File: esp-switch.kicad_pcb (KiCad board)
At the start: 2 copper layers, 50.8 x 50.8 mm, 29 parts, among them J1 Screw_Terminal_01x03, J2 Conn_01x04, J3 Screw_Terminal_01x03, J4 Conn_01x04, U1 ATTINY441-SSU, U2 ESP-01v090, U3 MOC3041M, U4 MOC3041M, U5 HLK-PM03

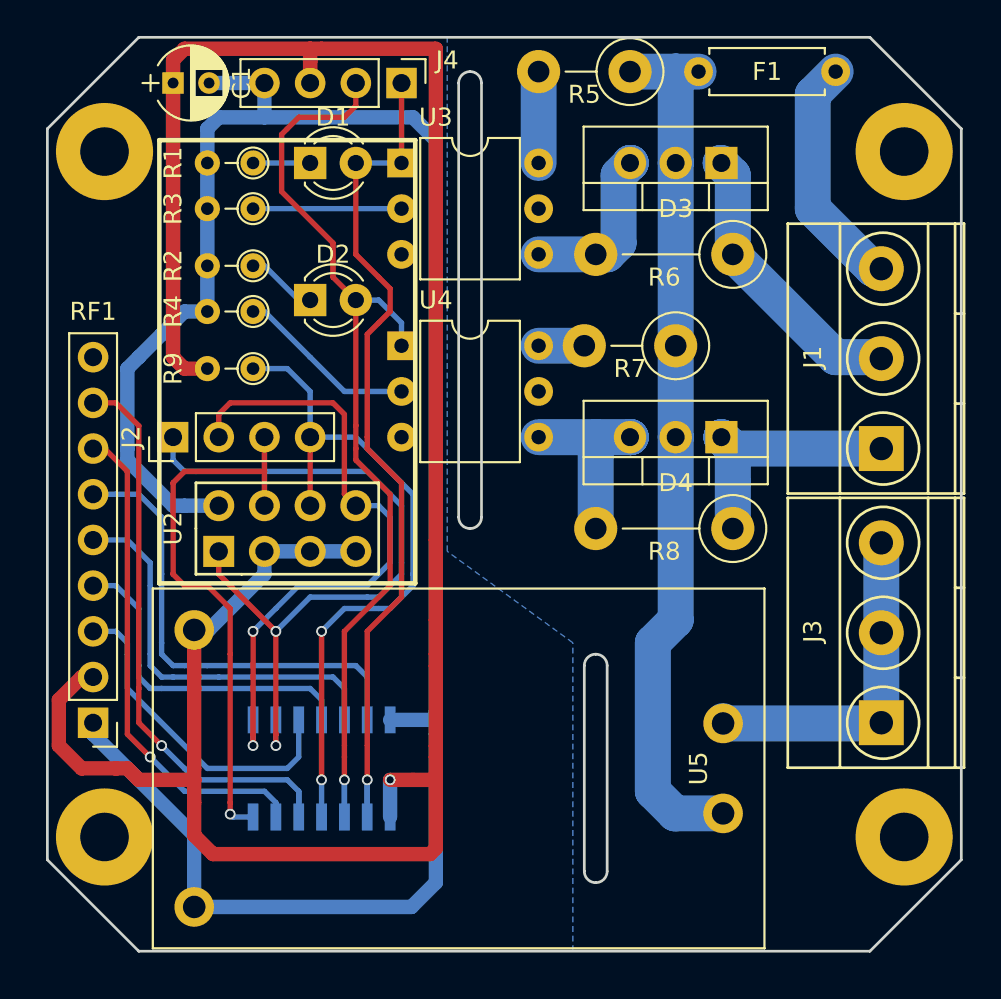
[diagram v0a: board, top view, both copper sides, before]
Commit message: V4 schematics
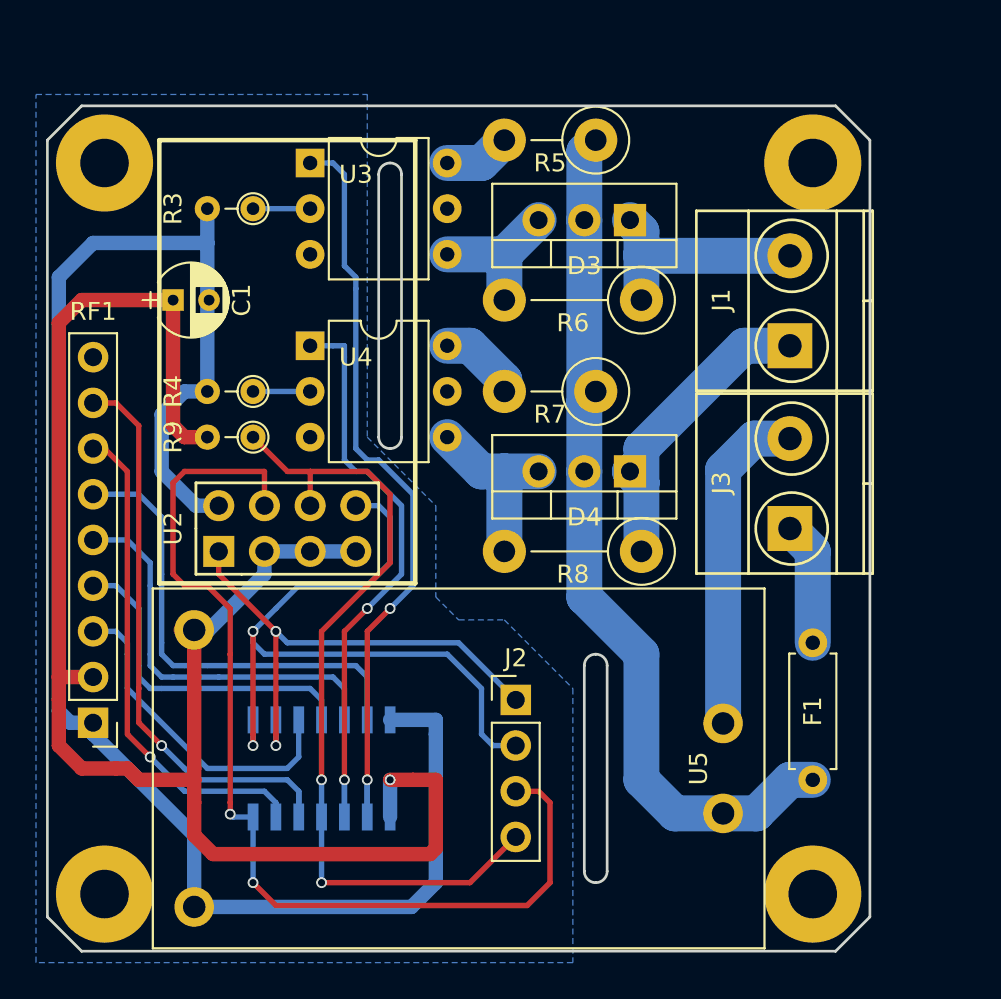
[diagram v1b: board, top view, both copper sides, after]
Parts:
- removed D1, D2: LED, LEDs:LED_D3.0mm
- removed J4: Conn_01x04, Pin_Headers:Pin_Header_Straight_1x04_Pitch2.54mm
- removed R1, R2: 470R, Resistors_THT:R_Axial_DIN0204_L3.6mm_D1.6mm_P2.54mm_Vertical
- D3, D4: value BT137 -> BTA08-600BW
- J1, J3: value Screw_Terminal_01x03 -> Screw_Terminal_01x02; footprint Connectors_Terminal_Blocks:TerminalBlock_Pheonix_MKDS1.5-3pol -> Connectors_Terminal_Blocks:TerminalBlock_Pheonix_MKDS1.5-2pol
- R3, R4: value 470R -> 150R
- U3, U4: value MOC3041M -> MOC3043M
- moved F1 39.9 mm to (215.9, 134.6), turned to 90 degrees
- moved J2 24.0 mm to (199.4, 130.2), turned to 0 degrees
- moved C1 12.1 mm to (180.3, 108.0)
- moved J3 11.9 mm to (214.6, 120.7)
- moved J1 7.65 mm to (214.6, 110.5)
- moved REF** 5.99 mm to (215.9, 141.0)
- moved D3 5.99 mm to (205.7, 103.5)
- moved R6 5.68 mm to (206.4, 108.0)
- moved D4 5.43 mm to (205.7, 117.5)
- moved R8 5.24 mm to (206.4, 121.9)
- moved R7 5.12 mm to (203.8, 113.0)
- moved REF** 5.12 mm to (215.9, 100.3)
- moved U3 5.08 mm to (188.0, 100.3)
- moved U4 5.08 mm to (188.0, 110.5)
- moved R4 4.45 mm to (184.8, 113.0)
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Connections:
- J3 pad 1: Net-(J3-Pad1) -> Net-(F1-Pad2)
- J3 pad 2: Net-(J3-Pad1) -> Net-(J3-Pad2)
- U5 pad 2: Net-(J3-Pad1) -> Net-(J3-Pad2)
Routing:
- net +3V3: track 135.4 -> 96.5 mm
- net Net-(J2-Pad3): track 31.0 -> 56.9 mm, vias 1 -> 2
- net GND: track 116.1 -> 93.9 mm
- net Net-(J4-Pad2): track 53.3 -> 33.2 mm, vias 1 -> 2
- net Net-(J3-Pad1): track 19.1 -> 0.00 mm
- net Net-(J3-Pad2): track 0.00 -> 18.7 mm
- net Net-(J2-Pad1): track 40.7 -> 28.5 mm
- net Net-(J2-Pad4): track 38.6 -> 46.5 mm
- net Net-(R4-Pad1): track 10.1 -> 3.18 mm
- net Net-(F1-Pad2): track 13.3 -> 6.88 mm
- net Net-(J4-Pad1): track 47.7 -> 42.3 mm, vias 1 -> 2
- net Net-(R3-Pad1): track 8.25 -> 3.18 mm
- net Net-(J2-Pad2): track 35.8 -> 40.8 mm
- net Net-(D2-Pad1): track 3.96 -> 0.00 mm
- net Net-(D1-Pad1): track 3.18 -> 0.00 mm
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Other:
- board size 50.8 x 50.8 mm -> 45.7 x 47 mm
- board text added: "L"
- board text added: "L1"
- board text added: "L2"
- board text added: "N"
- board text added: "© 2020 Foxel V4"
- board text removed: "© 2018 Foxel V3"
